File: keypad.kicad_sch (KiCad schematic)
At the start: 1 part, among them J7 KEYPAD_4X4

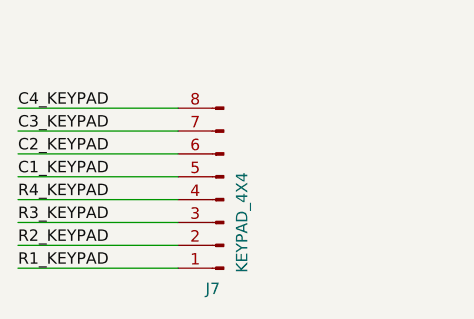
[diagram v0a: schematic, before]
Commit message: adad
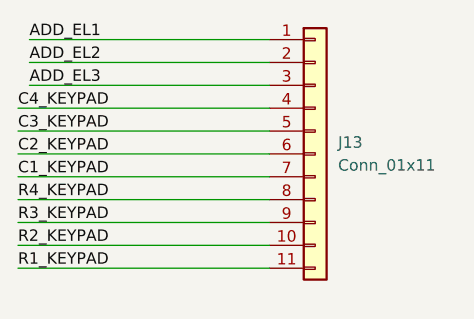
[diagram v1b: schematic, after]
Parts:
- removed J7: KEYPAD_4X4, symbol Connector:Conn_01x08_Pin
- added J13: Conn_01x11, symbol Connector_Generic:Conn_01x11
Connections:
- net C1_KEYPAD: now also J13.7 (Pin_7)
- net C2_KEYPAD: now also J13.6 (Pin_6)
- net C3_KEYPAD: now also J13.5 (Pin_5)
- net C4_KEYPAD: now also J13.4 (Pin_4)
- net R1_KEYPAD: now also J13.11 (Pin_11)
- net R2_KEYPAD: now also J13.10 (Pin_10)
- net R3_KEYPAD: now also J13.9 (Pin_9)
- net R4_KEYPAD: now also J13.8 (Pin_8)
- new net ADD_EL1: J13.1 (Pin_1)
- new net ADD_EL2: J13.2 (Pin_2)
- new net ADD_EL3: J13.3 (Pin_3)
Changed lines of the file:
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@@
 	(wire
 		(pts
-			(xy 68.58 46.99) (xy 86.36 46.99)
-		)
-		(stroke
-			(width 0)
-			(type default)
-		)
-	)
-	(wire
-		(pts
-			(xy 68.58 41.91) (xy 86.36 41.91)
-		)
-		(stroke
-			(width 0)
-			(type default)
-		)
-	)
-	(wire
-		(pts
-			(xy 68.58 57.15) (xy 86.36 57.15)
-		)
-		(stroke
-			(width 0)
-			(type default)
-		)
-	)
-	(wire
-		(pts
-			(xy 68.58 44.45) (xy 86.36 44.45)
-		)
-		(stroke
-			(width 0)
-			(type default)
-		)
-	)
-	(wire
-		(pts
-			(xy 68.58 52.07) (xy 86.36 52.07)
-		)
-		(stroke
-			(width 0)
-			(type default)
-		)
-	)
-	(wire
-		(pts
-			(xy 68.58 54.61) (xy 86.36 54.61)
-		)
-		(stroke
-			(width 0)
-			(type default)
-		)
-	)
-	(wire
-		(pts
-			(xy 68.58 49.53) (xy 86.36 49.53)
-		)
-		(stroke
-			(width 0)
-			(type default)
-		)
-	)
-	(wire
-		(pts
-			(xy 68.58 59.69) (xy 86.36 59.69)
-		)
-		(stroke
-			(width 0)
-			(type default)
+			(xy 68.58 46.99) (xy 96.52 46.99)
+		)
+		(stroke
+			(width 0)
+			(type default)
+		)
+	)
+	(wire
+		(pts
+			(xy 68.58 41.91) (xy 96.52 41.91)
+		)
+		(stroke
+			(width 0)
+			(type default)
+		)
+	)
+	(wire
+		(pts
+			(xy 69.85 34.29) (xy 96.52 34.29)
+		)
+		(stroke
+			(width 0)
+			(type default)
+		)
+	)
+	(wire
+		(pts
+			(xy 69.85 39.37) (xy 96.52 39.37)
+		)
+		(stroke
+			(width 0)
+			(type default)
+		)
+	)
+	(wire
+		(pts
+			(xy 68.58 57.15) (xy 96.52 57.15)
+		)
+		(stroke
+			(width 0)
+			(type default)
+		)
+	)
+	(wire
+		(pts
+			(xy 68.58 44.45) (xy 96.52 44.45)
+		)
+		(stroke
+			(width 0)
+			(type default)
+		)
+	)
+	(wire
+		(pts
+			(xy 69.85 36.83) (xy 96.52 36.83)
+		)
+		(stroke
+			(width 0)
+			(type default)
+		)
+	)
+	(wire
+		(pts
+			(xy 68.58 52.07) (xy 96.52 52.07)
+		)
+		(stroke
+			(width 0)
+			(type default)
+		)
+	)
+	(wire
+		(pts
+			(xy 68.58 54.61) (xy 96.52 54.61)
+		)
+		(stroke
+			(width 0)
+			(type default)
+		)
+	)
+	(wire
+		(pts
+			(xy 68.58 49.53) (xy 96.52 49.53)
+		)
+		(stroke
+			(width 0)
+			(type default)
+		)
+	)
+	(wire
+		(pts
+			(xy 68.58 59.69) (xy 96.52 59.69)
+		)
+		(stroke
+			(width 0)
+			(type default)
+		)
+	)
+	(label "ADD_EL1"
+		(at 69.85 34.29 0)
+		(fields_autoplaced yes)
+		(effects
+			(font
+				(size 1.27 1.27)
+			)
+			(justify left bottom)
+		)
+	)
+	(label "ADD_EL3"
+		(at 69.85 39.37 0)
+		(fields_autoplaced yes)
+		(effects
+			(font
+				(size 1.27 1.27)
+			)
+			(justify left bottom)
 		)
 	)
@@
 		)
 	)
+	(label "ADD_EL2"
+		(at 69.85 36.83 0)
+		(fields_autoplaced yes)
+		(effects
+			(font
+				(size 1.27 1.27)
+			)
+			(justify left bottom)
+		)
+	)
 	(label "R4_KEYPAD"
 		(at 68.58 52.07 0)
@@
 	)
 	(symbol
-		(lib_id "Connector:Conn_01x08_Pin")
-		(at 91.44 52.07 180)
+		(lib_id "Connector_Generic:Conn_01x11")
+		(at 101.6 46.99 0)
 		(unit 1)
 		(exclude_from_sim no)
@@
 		(on_board yes)
 		(dnp no)
-		(property "Reference" "J7"
-			(at 89.408 61.976 0)
-			(effects
-				(font
-					(size 1.27 1.27)
-				)
-				(justify right)
-			)
-		)
-		(property "Value" "KEYPAD_4X4"
-			(at 93.472 60.198 90)
-			(effects
-				(font
-					(size 1.27 1.27)
-				)
-				(justify right)
+		(fields_autoplaced yes)
+		(property "Reference" "J13"
+			(at 104.14 45.7199 0)
+			(effects
+				(font
+					(size 1.27 1.27)
+				)
+				(justify left)
+			)
+		)
+		(property "Value" "Conn_01x11"
+			(at 104.14 48.2599 0)
+			(effects
+				(font
+					(size 1.27 1.27)
+				)
+				(justify left)
 			)
 		)
 		(property "Footprint" ""
-			(at 91.44 52.07 0)
+			(at 101.6 46.99 0)
 			(effects
 				(font
@@
 		)
 		(property "Datasheet" "~"
-			(at 91.44 52.07 0)
+			(at 101.6 46.99 0)
 			(effects
 				(font
@@
 			)
 		)
-		(property "Description" "Generic connector, single row, 01x08, script generated"
-			(at 91.44 52.07 0)
+		(property "Description" "Generic connector, single row, 01x11, script generated (kicad-library-utils/schlib/autogen/connector/)"
+			(at 101.6 46.99 0)
 			(effects
 				(font
@@
 			)
 		)
+		(pin "3"
+		)
+		(pin "11"
+		)
+		(pin "7"
+		)
+		(pin "8"
+		)
 		(pin "4"
 		)
-		(pin "8"
-		)
-		(pin "7"
+		(pin "9"
 		)
 		(pin "5"
 		)
-		(pin "3"
+		(pin "6"
+		)
+		(pin "1"
 		)
 		(pin "2"
 		)
-		(pin "1"
-		)
-		(pin "6"
+		(pin "10"
 		)
 		(instances
 			(project ""
 				(path "/7e5ed2de-adc7-481a-a10e-7326381f5ab2/6da800c5-b029-4710-b0da-d69ee516648b"
-					(reference "J7")
+					(reference "J13")
 					(unit 1)
 				)

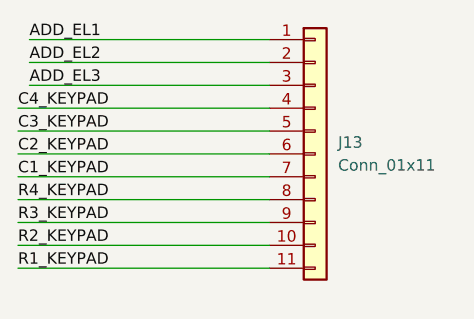
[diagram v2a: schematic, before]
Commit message: da
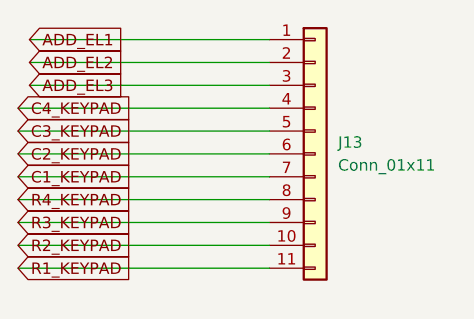
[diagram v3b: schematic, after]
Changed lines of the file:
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@@
 		)
 	)
-	(label "ADD_EL1"
+	(global_label "C3_KEYPAD"
+		(shape input)
+		(at 68.58 44.45 0)
+		(fields_autoplaced yes)
+		(effects
+			(font
+				(size 1.27 1.27)
+			)
+			(justify left)
+		)
+		(property "Intersheetrefs" "${INTERSHEET_REFS}"
+			(at 82.1485 44.45 0)
+			(effects
+				(font
+					(size 1.27 1.27)
+				)
+				(justify left)
+				(hide yes)
+			)
+		)
+	)
+	(global_label "ADD_EL1"
+		(shape input)
 		(at 69.85 34.29 0)
 		(fields_autoplaced yes)
@@
 				(size 1.27 1.27)
 			)
-			(justify left bottom)
-		)
-	)
-	(label "ADD_EL3"
+			(justify left)
+		)
+		(property "Intersheetrefs" "${INTERSHEET_REFS}"
+			(at 80.818 34.29 0)
+			(effects
+				(font
+					(size 1.27 1.27)
+				)
+				(justify left)
+				(hide yes)
+			)
+		)
+	)
+	(global_label "ADD_EL3"
+		(shape input)
 		(at 69.85 39.37 0)
 		(fields_autoplaced yes)
@@
 				(size 1.27 1.27)
 			)
-			(justify left bottom)
-		)
-	)
-	(label "R2_KEYPAD"
+			(justify left)
+		)
+		(property "Intersheetrefs" "${INTERSHEET_REFS}"
+			(at 80.818 39.37 0)
+			(effects
+				(font
+					(size 1.27 1.27)
+				)
+				(justify left)
+				(hide yes)
+			)
+		)
+	)
+	(global_label "R2_KEYPAD"
+		(shape input)
 		(at 68.58 57.15 0)
 		(fields_autoplaced yes)
@@
 				(size 1.27 1.27)
 			)
-			(justify left bottom)
-		)
-	)
-	(label "R3_KEYPAD"
+			(justify left)
+		)
+		(property "Intersheetrefs" "${INTERSHEET_REFS}"
+			(at 82.1485 57.15 0)
+			(effects
+				(font
+					(size 1.27 1.27)
+				)
+				(justify left)
+				(hide yes)
+			)
+		)
+	)
+	(global_label "R4_KEYPAD"
+		(shape input)
+		(at 68.58 52.07 0)
+		(fields_autoplaced yes)
+		(effects
+			(font
+				(size 1.27 1.27)
+			)
+			(justify left)
+		)
+		(property "Intersheetrefs" "${INTERSHEET_REFS}"
+			(at 82.1485 52.07 0)
+			(effects
+				(font
+					(size 1.27 1.27)
+				)
+				(justify left)
+				(hide yes)
+			)
+		)
+	)
+	(global_label "C4_KEYPAD"
+		(shape input)
+		(at 68.58 41.91 0)
+		(fields_autoplaced yes)
+		(effects
+			(font
+				(size 1.27 1.27)
+			)
+			(justify left)
+		)
+		(property "Intersheetrefs" "${INTERSHEET_REFS}"
+			(at 82.1485 41.91 0)
+			(effects
+				(font
+					(size 1.27 1.27)
+				)
+				(justify left)
+				(hide yes)
+			)
+		)
+	)
+	(global_label "C1_KEYPAD"
+		(shape input)
+		(at 68.58 49.53 0)
+		(fields_autoplaced yes)
+		(effects
+			(font
+				(size 1.27 1.27)
+			)
+			(justify left)
+		)
+		(property "Intersheetrefs" "${INTERSHEET_REFS}"
+			(at 82.1485 49.53 0)
+			(effects
+				(font
+					(size 1.27 1.27)
+				)
+				(justify left)
+				(hide yes)
+			)
+		)
+	)
+	(global_label "R1_KEYPAD"
+		(shape input)
+		(at 68.58 59.69 0)
+		(fields_autoplaced yes)
+		(effects
+			(font
+				(size 1.27 1.27)
+			)
+			(justify left)
+		)
+		(property "Intersheetrefs" "${INTERSHEET_REFS}"
+			(at 82.1485 59.69 0)
+			(effects
+				(font
+					(size 1.27 1.27)
+				)
+				(justify left)
+				(hide yes)
+			)
+		)
+	)
+	(global_label "C2_KEYPAD"
+		(shape input)
+		(at 68.58 46.99 0)
+		(fields_autoplaced yes)
+		(effects
+			(font
+				(size 1.27 1.27)
+			)
+			(justify left)
+		)
+		(property "Intersheetrefs" "${INTERSHEET_REFS}"
+			(at 82.1485 46.99 0)
+			(effects
+				(font
+					(size 1.27 1.27)
+				)
+				(justify left)
+				(hide yes)
+			)
+		)
+	)
+	(global_label "ADD_EL2"
+		(shape input)
+		(at 69.85 36.83 0)
+		(fields_autoplaced yes)
+		(effects
+			(font
+				(size 1.27 1.27)
+			)
+			(justify left)
+		)
+		(property "Intersheetrefs" "${INTERSHEET_REFS}"
+			(at 80.818 36.83 0)
+			(effects
+				(font
+					(size 1.27 1.27)
+				)
+				(justify left)
+				(hide yes)
+			)
+		)
+	)
+	(global_label "R3_KEYPAD"
+		(shape input)
 		(at 68.58 54.61 0)
 		(fields_autoplaced yes)
@@
 				(size 1.27 1.27)
 			)
-			(justify left bottom)
-		)
-	)
-	(label "R1_KEYPAD"
-		(at 68.58 59.69 0)
-		(fields_autoplaced yes)
-		(effects
-			(font
-				(size 1.27 1.27)
-			)
-			(justify left bottom)
-		)
-	)
-	(label "C1_KEYPAD"
-		(at 68.58 49.53 0)
-		(fields_autoplaced yes)
-		(effects
-			(font
-				(size 1.27 1.27)
-			)
-			(justify left bottom)
-		)
-	)
-	(label "C4_KEYPAD"
-		(at 68.58 41.91 0)
-		(fields_autoplaced yes)
-		(effects
-			(font
-				(size 1.27 1.27)
-			)
-			(justify left bottom)
-		)
-	)
-	(label "C3_KEYPAD"
-		(at 68.58 44.45 0)
-		(fields_autoplaced yes)
-		(effects
-			(font
-				(size 1.27 1.27)
-			)
-			(justify left bottom)
-		)
-	)
-	(label "C2_KEYPAD"
-		(at 68.58 46.99 0)
-		(fields_autoplaced yes)
-		(effects
-			(font
-				(size 1.27 1.27)
-			)
-			(justify left bottom)
-		)
-	)
-	(label "ADD_EL2"
-		(at 69.85 36.83 0)
-		(fields_autoplaced yes)
-		(effects
-			(font
-				(size 1.27 1.27)
-			)
-			(justify left bottom)
-		)
-	)
-	(label "R4_KEYPAD"
-		(at 68.58 52.07 0)
-		(fields_autoplaced yes)
-		(effects
-			(font
-				(size 1.27 1.27)
-			)
-			(justify left bottom)
-		)
-	)
+			(justify left)
+		)
+		(property "Intersheetrefs" "${INTERSHEET_REFS}"
+			(at 82.1485 54.61 0)
+			(effects
+				(font
+					(size 1.27 1.27)
+				)
+				(justify left)
+				(hide yes)
+			)
+		)
+	)
